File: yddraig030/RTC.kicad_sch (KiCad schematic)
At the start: 9 parts

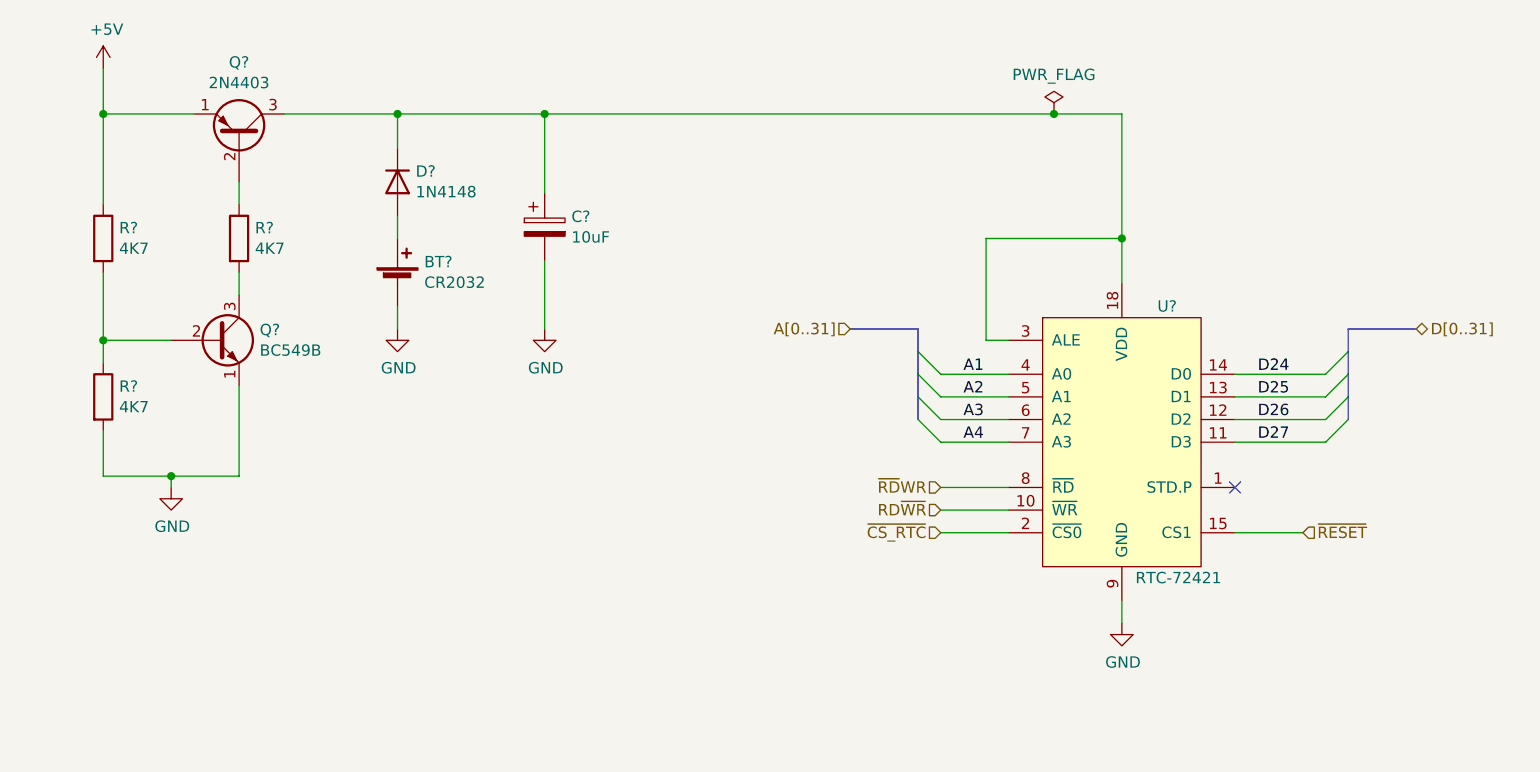
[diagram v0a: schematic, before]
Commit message: Updated 030 design files
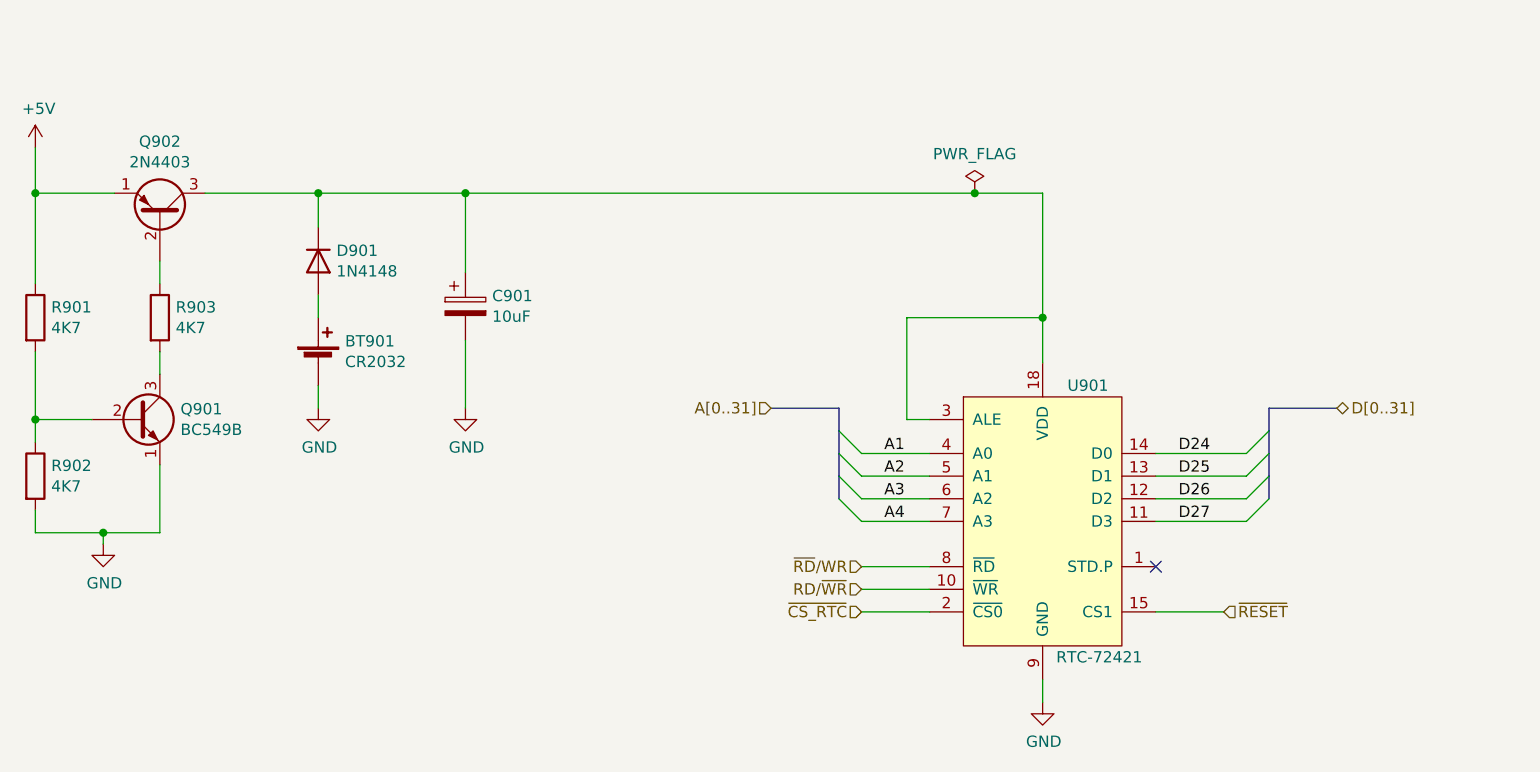
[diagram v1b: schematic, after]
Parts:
- removed BT?: CR2032, Battery:BatteryHolder_Keystone_103_1x20mm, symbol Device:Battery_Cell
- removed C?: 10uF, Capacitor_THT:CP_Radial_D5.0mm_P2.50mm, symbol Device:CP
- removed D?: 1N4148, Diode_THT:D_DO-35_SOD27_P7.62mm_Horizontal, symbol Diode:1N4148
- removed Q?: BC549B, Package_TO_SOT_THT:TO-92, symbol Device:Q_NPN_EBC
- removed Q?: 2N4403, Package_TO_SOT_THT:TO-92, symbol Device:Q_PNP_EBC
- removed R? (x3): 4K7, Resistor_THT:R_Axial_DIN0207_L6.3mm_D2.5mm_P10.16mm_Horizontal, symbol Device:R
- removed U?: RTC-72421, Package_DIP:DIP-18_W7.62mm_Socket, symbol Ddraig:RTC-72421
- added BT901: CR2032, Battery:BatteryHolder_Keystone_103_1x20mm, symbol Device:Battery_Cell
- added C901: 10uF, Capacitor_THT:CP_Radial_D5.0mm_P2.50mm, symbol Device:C_Polarized
- added D901: 1N4148, Diode_THT:D_DO-35_SOD27_P7.62mm_Horizontal, symbol Diode:1N4148
- added Q901: BC549B, Package_TO_SOT_THT:TO-92, symbol Device:Q_NPN_EBC
- added Q902: 2N4403, Package_TO_SOT_THT:TO-92, symbol Device:Q_PNP_EBC
- added R901, R902, R903: 4K7, Resistor_THT:R_Axial_DIN0207_L6.3mm_D2.5mm_P10.16mm_Horizontal, symbol Device:R
- added U901: RTC-72421, Package_DIP:DIP-18_W7.62mm_Socket, symbol Ddraig:RTC-72421
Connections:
- net +5V: now also Q902.1 (E), R901.1
- net A1: now also U901.4 (A0)
- net A2: now also U901.5 (A1)
- net A3: now also U901.6 (A2)
- net A4: now also U901.7 (A3)
- net D24: now also U901.14 (D0)
- net D25: now also U901.13 (D1)
- net D26: now also U901.12 (D2)
- net D27: now also U901.11 (D3)
- net GND: now also BT901.2 (-), C901.2, Q901.1 (E), R902.2, U901.9 (GND)
- net ~{CS_RTC}: now also U901.2 (~{CS0})
- net ~{RESET}: now also U901.15 (CS1)
- new net: C901.1, D901.1 (K), Q902.3 (C), U901.18 (VDD), U901.3 (ALE)
- new net: Q901.2 (B), R901.2, R902.1
- new net: Q901.3 (C), R903.2
- new net: Q902.2 (B), R903.1
- new net: BT901.1 (+), D901.2 (A)
- new net RD/~{WR}: U901.10 (~{WR})
- new net ~{RD}/WR: U901.8 (~{RD})
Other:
- company: (none) -> Stephen Moody
- title: (none) -> Y Ddraig Fawr
